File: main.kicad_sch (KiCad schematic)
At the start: 34 parts, among them J1 USB_C_Receptacle_USB2.0_14P, SW1 SW_PUSH, SW2 SW_PUSH, SW3 SW_PUSH, SW4 SW_PUSH, SW5 SW_PUSH, U1 NCP1117-3.3_SOT223, U2 RP2040, U3 W25Q128JVS, Y1 ABM8-272-T3

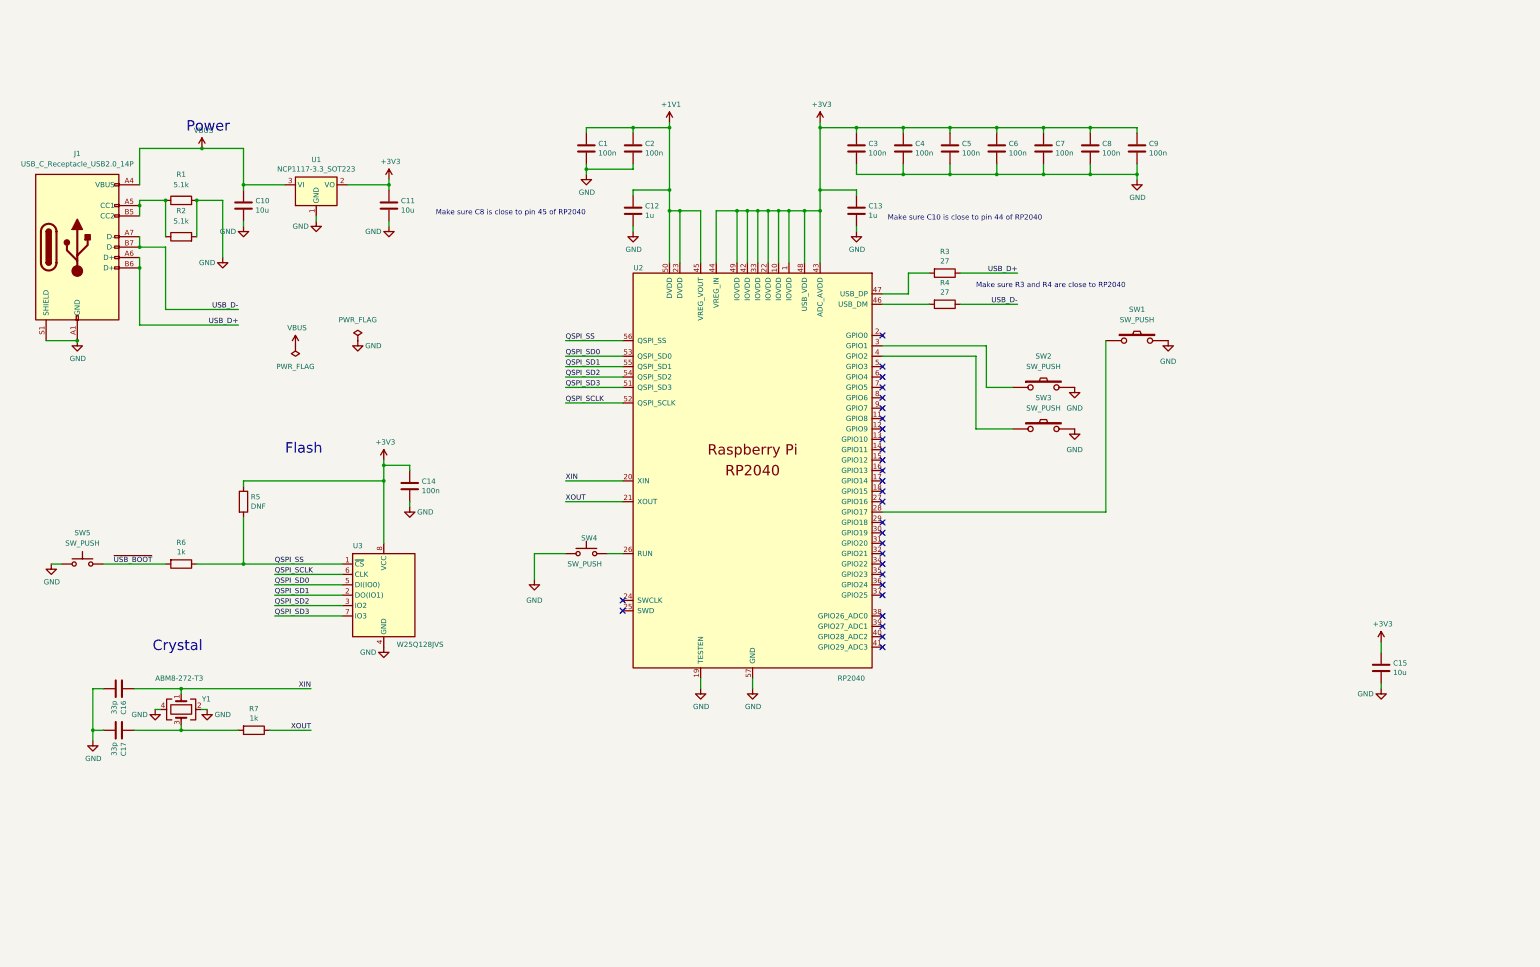
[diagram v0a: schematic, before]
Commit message: :sparkles: (all) prepare fab
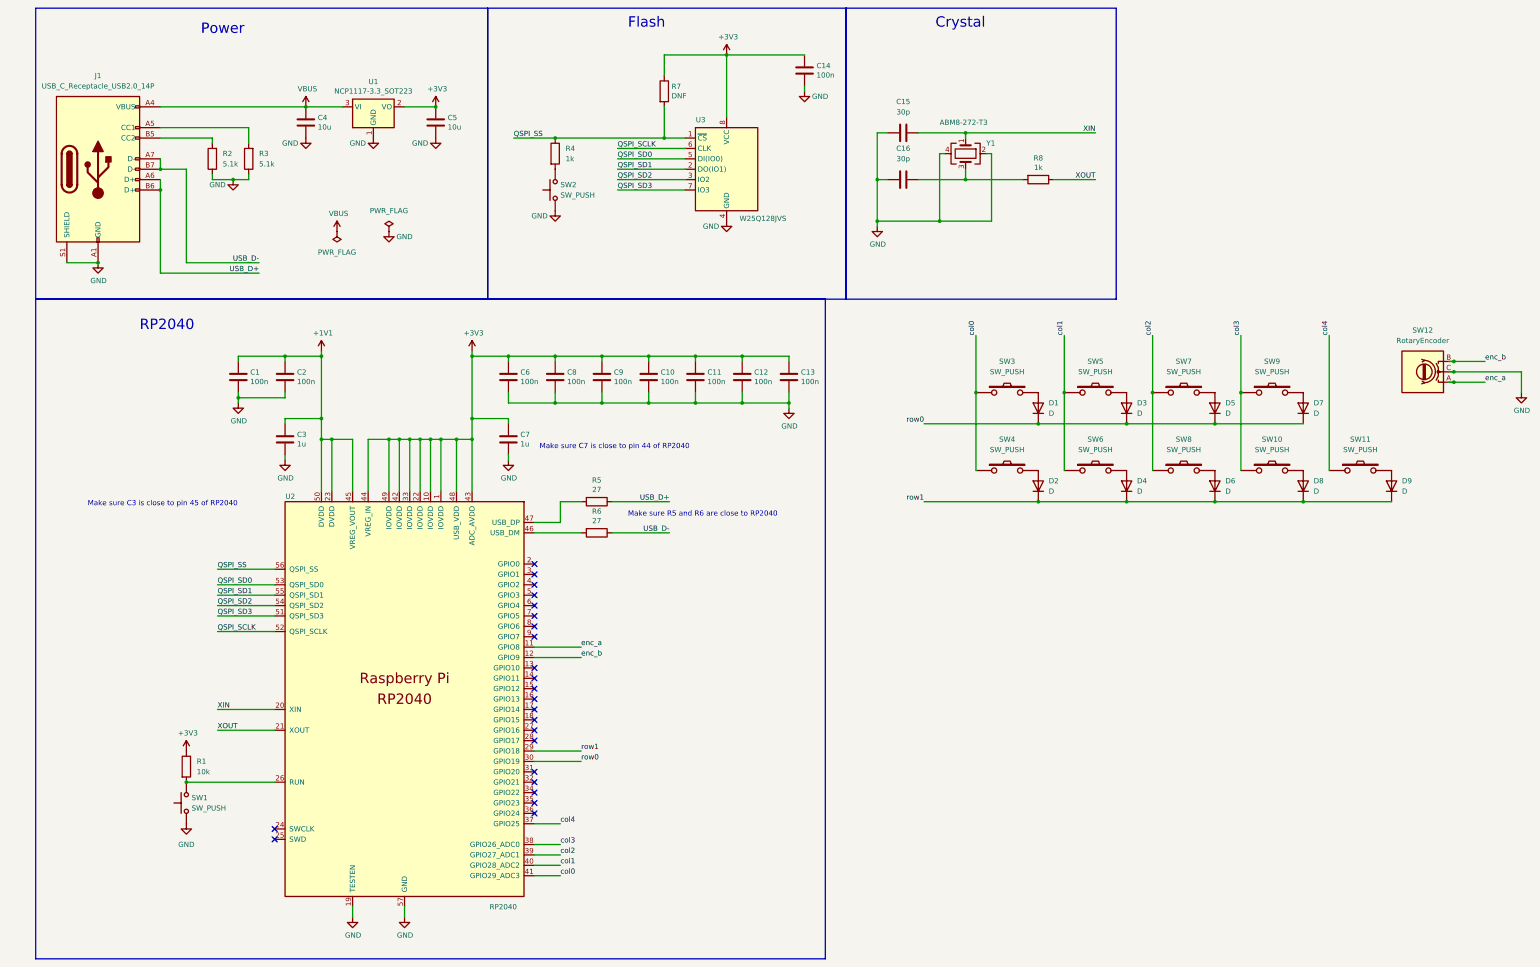
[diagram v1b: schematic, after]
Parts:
- removed C10: 10u, Capacitor_SMD:C_0805_2012Metric, symbol Device:C
- removed C17: 33p, Capacitor_SMD:C_0402_1005Metric, symbol Device:C
- removed R6: 1k, Resistor_SMD:R_0402_1005Metric, symbol Device:R
- removed SW1, SW2: SW_PUSH, kamo3_footprint:SW_CherryMX_Hotswap_1.25u, symbol kbd:SW_PUSH
- removed SW4: SW_PUSH, kamo3_footprint:Tact_Switch_5.1_5.1mm_SMD, symbol kamo3_symbol:SW_Push_4pin
- added C4: 10u, Capacitor_SMD:C_0805_2012Metric, symbol Device:C
- added D1, D2, D3, D4, D5, D6, D7, D8, D9: D, kamo3_footprint:Diode_SOD123, symbol Device:D
- added R1: 10k, Resistor_SMD:R_0402_1005Metric, symbol Device:R
- added R4: 1k, Resistor_SMD:R_0402_1005Metric, symbol Device:R
- added SW1: SW_PUSH, kamo3_footprint:Tact_Switch_5.1_5.1mm_SMD, symbol kamo3_symbol:SW_Push_4pin
- added SW10, SW4, SW5, SW6, SW7, SW8, SW9: SW_PUSH, kamo3_footprint:SW_ChocV1_Hotswap_1.0u, symbol kbd:SW_PUSH
- added SW11: SW_PUSH, kamo3_footprint:SW_ChocV1_Hotswap_1.50u, symbol kbd:SW_PUSH
- added SW12: RotaryEncoder, Rotary_Encoder:RotaryEncoder_Alps_EC12E_Vertical_H20mm, symbol Device:RotaryEncoder
- C15: value 10u -> 30p; footprint Capacitor_SMD:C_0805_2012Metric -> Capacitor_SMD:C_0603_1608Metric; LCSC C15850 -> C1658
- C16: value 33p -> 30p; footprint Capacitor_SMD:C_0402_1005Metric -> Capacitor_SMD:C_0603_1608Metric; LCSC C1562 -> C1658
- R5: renamed from R3; footprint Resistor_SMD:R_0402_1005Metric -> Resistor_SMD:R_0603_1608Metric; LCSC C321419 -> C25190
- R6: renamed from R4; footprint Resistor_SMD:R_0402_1005Metric -> Resistor_SMD:R_0603_1608Metric; LCSC C321419 -> C25190
- R7: renamed from R5; LCSC C17168 -> (none)
- SW3: footprint kamo3_footprint:SW_CherryMX_Hotswap_1.00u -> kamo3_footprint:SW_ChocV1_Hotswap_1.0u
- renumbered C6 to C10, C7 to C11, C8 to C12, C9 to C13, C12 to C3, C11 to C5, C3 to C6, C13 to C7, C4 to C8, C5 to C9, R1 to R3, R7 to R8, SW5 to SW2
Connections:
- net +3V3: now also R1.1; no longer C15.1
- net GND: now also C15.1, C16.1, R2.1, R3.1, C4.2, SW1.1, SW1.2, SW12.C; no longer C15.2, C16.2, R2.2, R3.2, SW3.2
- net QSPI_SS: now also R4.1
- net VBUS: now also C4.1
- net XIN: now also C15.2; no longer C16.1
- net at R8.2, Y1.3: now also C16.2
- net at U2.4 (GPIO2): no longer SW3.1
- net at U2.26 (RUN): now also R1.2, SW1.3, SW1.4
- net enc_a: now reaches U2.11 (GPIO8)
- net enc_a: now also SW12.A
- net enc_b: now reaches U2.12 (GPIO9)
- net enc_b: now also SW12.B
- net row1: now reaches U2.29 (GPIO18)
- net row1: now also D2.1 (K), D4.1 (K), D6.1 (K), D8.1 (K), D9.1 (K)
- net row0: now reaches U2.30 (GPIO19)
- net row0: now also D1.1 (K), D3.1 (K), D5.1 (K), D7.1 (K)
- net col4: now reaches U2.37 (GPIO25)
- net col4: now also SW11.1
- net col3: now reaches U2.38 (GPIO26_ADC0)
- net col3: now also SW10.1, SW9.1
- net col2: now reaches U2.39 (GPIO27_ADC1)
- net col2: now also SW7.1, SW8.1
- net col1: now reaches U2.40 (GPIO28_ADC2)
- net col1: now also SW5.1, SW6.1
- net col0: now reaches U2.41 (GPIO29_ADC3)
- net col0: now also SW3.1, SW4.1
- net ~{USB_BOOT}: no longer names the net of SW2.3, SW2.4
- net ~{USB_BOOT}: now also R4.2
- new net: D3.2 (A), SW5.2
- new net: D5.2 (A), SW7.2
- new net: D2.2 (A), SW4.2
- new net: D7.2 (A), SW9.2
- new net: D6.2 (A), SW8.2
- new net: J1.B5 (CC2), R2.2
- new net: D8.2 (A), SW10.2
- new net: J1.A5 (CC1), R3.2
- new net: D1.2 (A), SW3.2
- new net: D4.2 (A), SW6.2
- new net: D9.2 (A), SW11.2
- no-connect marks 29 -> 23
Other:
- note added: "Make sure C3 is close to pin 45 of RP2040"
- note added: "Make sure C7 is close to pin 44 of RP2040"
- note added: "Make sure R5 and R6 are close to RP2040"
- note added: "RP2040"
- note removed: "Make sure C10 is close to pin 44 of RP2040"
- note removed: "Make sure C8 is close to pin 45 of RP2040"
- note removed: "Make sure R3 and R4 are close to RP2040"
- moved on the sheet: C1, C10, C11, C12, C13, C2, C3, C5, C6, C7, C8, C9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
